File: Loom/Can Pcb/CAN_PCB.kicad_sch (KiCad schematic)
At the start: 28 parts, among them J1 Conn_01x02, J12 Conn_01x03, J15 Conn_01x03, J16 Conn_01x03, J2 Conn_01x05_Pin, J4 Conn_01x02, J5 Conn_01x03, U2 MCP2551-I-P, U4 TL780-05KCS, Y1 Crystal

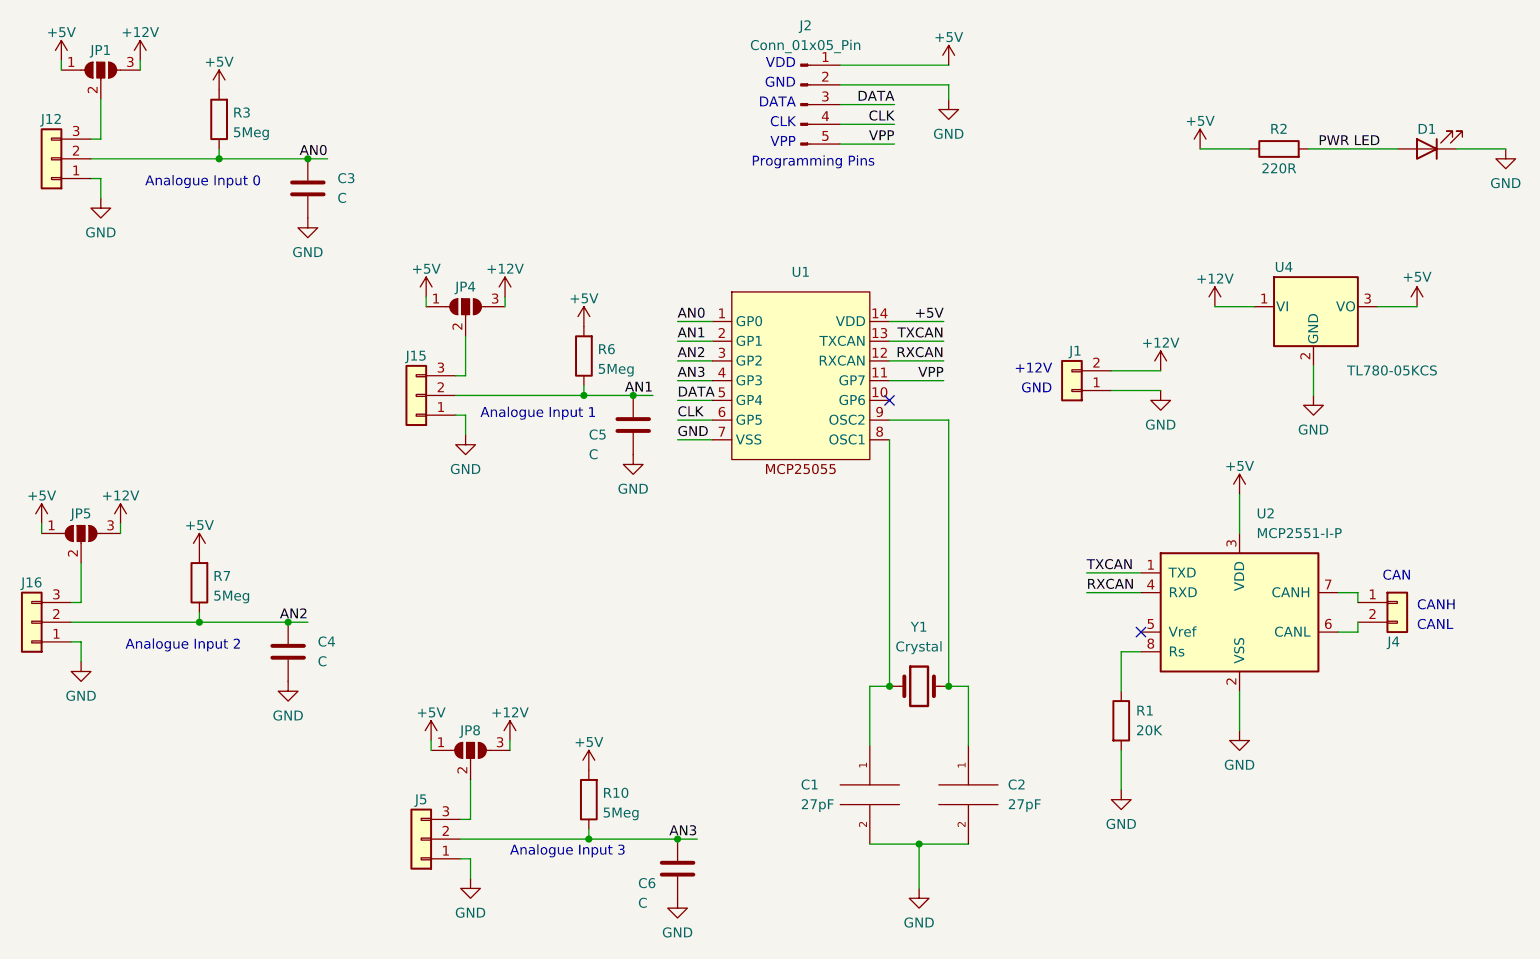
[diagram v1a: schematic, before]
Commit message: Revert "Merge branch 'CAN_PCB' of https://github.com/Full-Blue-Racing/FBR24-Electronics into CAN_PCB"
This reverts commit f7426b5fd5c3026a458d075125f69338a8895489, reversing
changes made to b85a40d8a8d15d08b24989522968470fc8db4cd4.
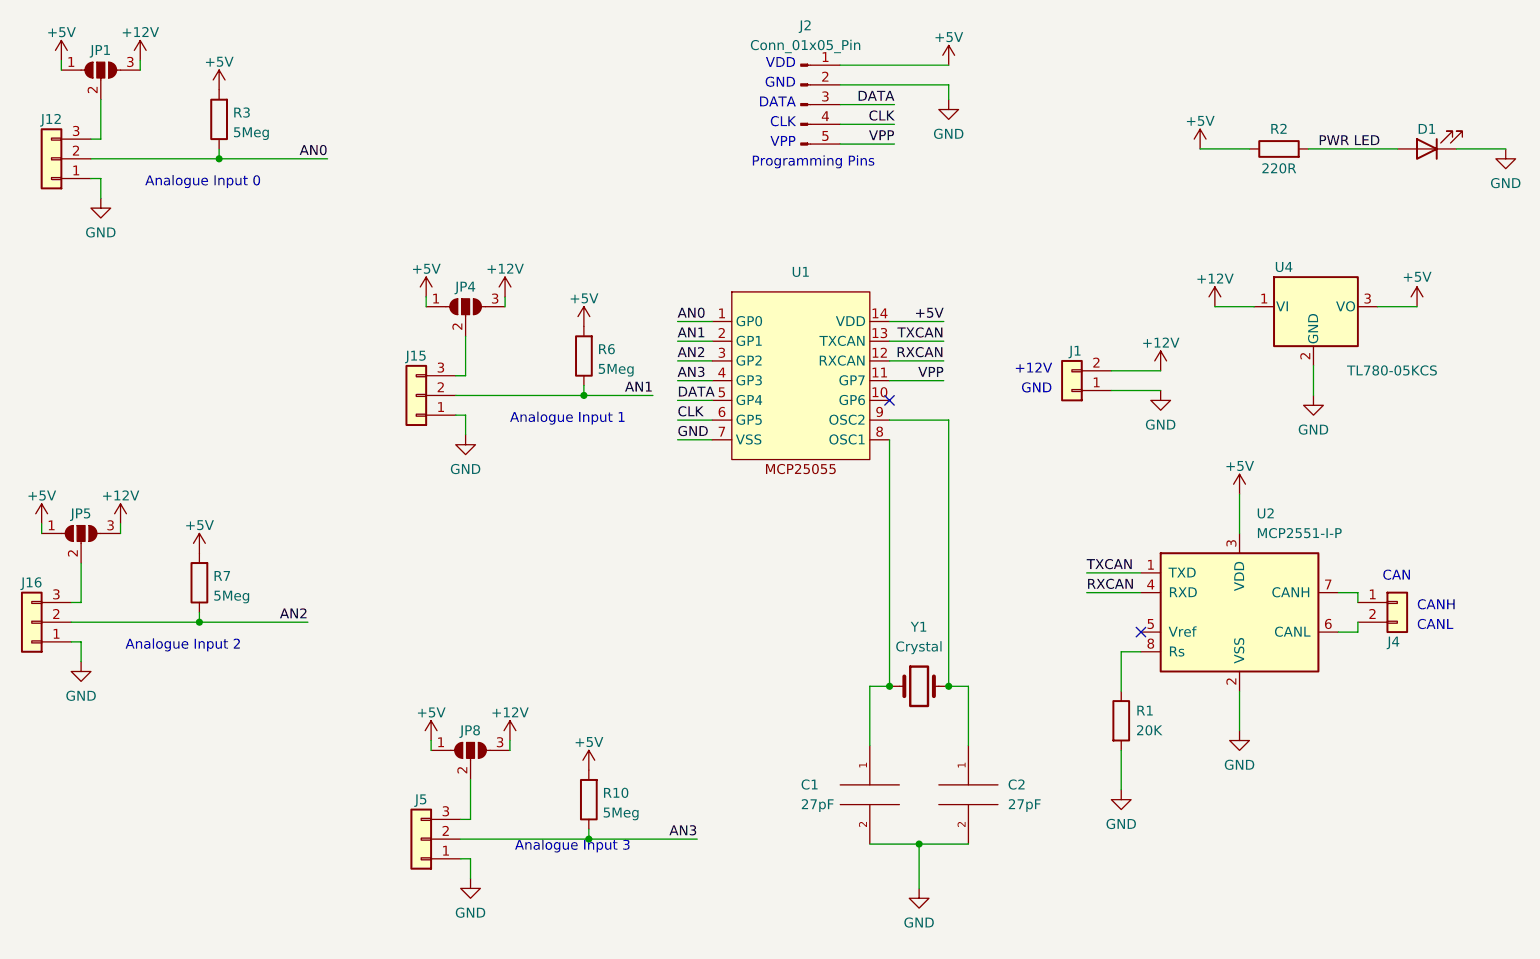
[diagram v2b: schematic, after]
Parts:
- removed C3, C4, C5, C6: C, Capacitor_THT:C_Disc_D4.7mm_W2.5mm_P5.00mm, symbol Device:C
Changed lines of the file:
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@@
     (title "Can Adapeter PCB")
   )
-  (junction (at 100.965 122.555) (diameter 0) (color 0 0 0 0)
-  )
   (junction (at 39.37 94.615) (diameter 0) (color 0 0 0 0)
   )
-  (junction (at 50.8 94.615) (diameter 0) (color 0 0 0 0)
-  )
   (junction (at 88.9 65.405) (diameter 0) (color 0 0 0 0)
   )
@@
   (junction (at 135.89 102.87) (diameter 0) (color 0 0 0 0)
   )
-  (junction (at 95.25 65.405) (diameter 0) (color 0 0 0 0)
-  )
   (junction (at 132.08 123.19) (diameter 0) (color 0 0 0 0)
-  )
-  (junction (at 53.34 34.925) (diameter 0) (color 0 0 0 0)
   )
   (junction (at 41.91 34.925) (diameter 0) (color 0 0 0 0)
@@
     (stroke (width 0) (type default))
   )
-  (wire (pts (xy 100.965 122.555) (xy 103.505 122.555))
-    (stroke (width 0) (type default))
-  )
   (wire (pts (xy 156.845 64.77) (xy 163.195 64.77))
     (stroke (width 0) (type default))
   )
-  (wire (pts (xy 95.25 65.405) (xy 97.79 65.405))
-    (stroke (width 0) (type default))
-  )
   (wire (pts (xy 100.965 68.58) (xy 105.41 68.58))
     (stroke (width 0) (type default))
@@
     (stroke (width 0) (type default))
   )
-  (wire (pts (xy 39.37 94.615) (xy 50.8 94.615))
+  (wire (pts (xy 39.37 94.615) (xy 53.34 94.615))
     (stroke (width 0) (type default))
   )
@@
     (stroke (width 0) (type default))
   )
-  (wire (pts (xy 88.9 65.405) (xy 95.25 65.405))
+  (wire (pts (xy 88.9 65.405) (xy 97.79 65.405))
     (stroke (width 0) (type default))
   )
@@
     (stroke (width 0) (type default))
   )
-  (wire (pts (xy 50.8 94.615) (xy 53.34 94.615))
-    (stroke (width 0) (type default))
-  )
   (wire (pts (xy 182.245 33.655) (xy 193.675 33.655))
     (stroke (width 0) (type default))
@@
     (stroke (width 0) (type default))
   )
-  (wire (pts (xy 53.34 34.925) (xy 55.88 34.925))
-    (stroke (width 0) (type default))
-  )
   (wire (pts (xy 121.92 30.48) (xy 128.905 30.48))
     (stroke (width 0) (type default))
@@
     (stroke (width 0) (type default))
   )
-  (wire (pts (xy 41.91 34.925) (xy 53.34 34.925))
-    (stroke (width 0) (type default))
-  )
-  (wire (pts (xy 89.535 122.555) (xy 100.965 122.555))
+  (wire (pts (xy 41.91 34.925) (xy 55.88 34.925))
+    (stroke (width 0) (type default))
+  )
+  (wire (pts (xy 89.535 122.555) (xy 103.505 122.555))
     (stroke (width 0) (type default))
   )
@@
     (effects (font (size 1.27 1.27)) (justify left bottom))
   )
-  (text "Analogue Input 3\n\n" (at 79.375 127 0)
+  (text "Analogue Input 3\n\n" (at 80.01 126.365 0)
     (effects (font (size 1.27 1.27)) (justify left bottom))
   )
@@
     (effects (font (size 1.27 1.27)) (justify right bottom))
   )
-  (text "Analogue Input 1\n" (at 75.565 68.58 0)
+  (text "Analogue Input 1\n" (at 79.375 69.215 0)
     (effects (font (size 1.27 1.27)) (justify left bottom))
   )
@@
     )
   )
-  (symbol (lib_id "Device:C") (at 95.25 69.215 0) (unit 1)
-    (in_bom yes) (on_board yes) (dnp no)
-    (property "Reference" "C5" (at 89.535 70.485 0)
-      (effects (font (size 1.27 1.27)) (justify left))
-    )
-    (property "Value" "C" (at 89.535 73.025 0)
-      (effects (font (size 1.27 1.27)) (justify left))
-    )
-    (property "Footprint" "Capacitor_THT:C_Disc_D4.7mm_W2.5mm_P5.00mm" (at 96.2152 73.025 0)
-      (effects (font (size 1.27 1.27)) hide)
-    )
-    (property "Datasheet" "~" (at 95.25 69.215 0)
-      (effects (font (size 1.27 1.27)) hide)
-    )
-    (pin "1")
-    (pin "2")
-    (instances
-      (project "CAN_PCB"
-        (path "/10118a9c-eb72-4c5f-b0c0-2b860c31ebad"
-          (reference "C5") (unit 1)
-        )
-      )
-    )
-  )
   (symbol (lib_id "power:+12V") (at 170.18 53.975 0) (unit 1)
     (in_bom yes) (on_board yes) (dnp no) (fields_autoplaced)
@@
     )
   )
-  (symbol (lib_id "power:GND") (at 53.34 42.545 0) (unit 1)
-    (in_bom yes) (on_board yes) (dnp no) (fields_autoplaced)
-    (property "Reference" "#PWR018" (at 53.34 48.895 0)
-      (effects (font (size 1.27 1.27)) hide)
-    )
-    (property "Value" "GND" (at 53.34 46.99 0)
-      (effects (font (size 1.27 1.27)))
-    )
-    (property "Footprint" "" (at 53.34 42.545 0)
-      (effects (font (size 1.27 1.27)) hide)
-    )
-    (property "Datasheet" "" (at 53.34 42.545 0)
-      (effects (font (size 1.27 1.27)) hide)
-    )
-    (pin "1")
-    (instances
-      (project "CAN_PCB"
-        (path "/10118a9c-eb72-4c5f-b0c0-2b860c31ebad"
-          (reference "#PWR018") (unit 1)
-        )
-      )
-    )
-  )
-  (symbol (lib_id "Device:C") (at 100.965 126.365 0) (unit 1)
-    (in_bom yes) (on_board yes) (dnp no)
-    (property "Reference" "C6" (at 95.885 128.27 0)
-      (effects (font (size 1.27 1.27)) (justify left))
-    )
-    (property "Value" "C" (at 95.885 130.81 0)
-      (effects (font (size 1.27 1.27)) (justify left))
-    )
-    (property "Footprint" "Capacitor_THT:C_Disc_D4.7mm_W2.5mm_P5.00mm" (at 101.9302 130.175 0)
-      (effects (font (size 1.27 1.27)) hide)
-    )
-    (property "Datasheet" "~" (at 100.965 126.365 0)
-      (effects (font (size 1.27 1.27)) hide)
-    )
-    (pin "1")
-    (pin "2")
-    (instances
-      (project "CAN_PCB"
-        (path "/10118a9c-eb72-4c5f-b0c0-2b860c31ebad"
-          (reference "C6") (unit 1)
-        )
-      )
-    )
-  )
   (symbol (lib_id "power:+12V") (at 31.75 22.225 0) (unit 1)
     (in_bom yes) (on_board yes) (dnp no) (fields_autoplaced)
@@
         (path "/10118a9c-eb72-4c5f-b0c0-2b860c31ebad"
           (reference "#PWR025") (unit 1)
-        )
-      )
-    )
-  )
-  (symbol (lib_id "power:GND") (at 50.8 102.235 0) (unit 1)
-    (in_bom yes) (on_board yes) (dnp no) (fields_autoplaced)
-    (property "Reference" "#PWR019" (at 50.8 108.585 0)
-      (effects (font (size 1.27 1.27)) hide)
-    )
-    (property "Value" "GND" (at 50.8 106.68 0)
-      (effects (font (size 1.27 1.27)))
-    )
-    (property "Footprint" "" (at 50.8 102.235 0)
-      (effects (font (size 1.27 1.27)) hide)
-    )
-    (property "Datasheet" "" (at 50.8 102.235 0)
-      (effects (font (size 1.27 1.27)) hide)
-    )
-    (pin "1")
-    (instances
-      (project "CAN_PCB"
-        (path "/10118a9c-eb72-4c5f-b0c0-2b860c31ebad"
-          (reference "#PWR019") (unit 1)
-        )
-      )
-    )
-  )
-  (symbol (lib_id "power:GND") (at 95.25 73.025 0) (unit 1)
-    (in_bom yes) (on_board yes) (dnp no) (fields_autoplaced)
-    (property "Reference" "#PWR017" (at 95.25 79.375 0)
-      (effects (font (size 1.27 1.27)) hide)
-    )
-    (property "Value" "GND" (at 95.25 77.47 0)
-      (effects (font (size 1.27 1.27)))
-    )
-    (property "Footprint" "" (at 95.25 73.025 0)
-      (effects (font (size 1.27 1.27)) hide)
-    )
-    (property "Datasheet" "" (at 95.25 73.025 0)
-      (effects (font (size 1.27 1.27)) hide)
-    )
-    (pin "1")
-    (instances
-      (project "CAN_PCB"
-        (path "/10118a9c-eb72-4c5f-b0c0-2b860c31ebad"
-          (reference "#PWR017") (unit 1)
-        )
-      )
-    )
-  )
-  (symbol (lib_id "power:GND") (at 100.965 130.175 0) (unit 1)
-    (in_bom yes) (on_board yes) (dnp no) (fields_autoplaced)
-    (property "Reference" "#PWR016" (at 100.965 136.525 0)
-      (effects (font (size 1.27 1.27)) hide)
-    )
-    (property "Value" "GND" (at 100.965 134.62 0)
-      (effects (font (size 1.27 1.27)))
-    )
-    (property "Footprint" "" (at 100.965 130.175 0)
-      (effects (font (size 1.27 1.27)) hide)
-    )
-    (property "Datasheet" "" (at 100.965 130.175 0)
-      (effects (font (size 1.27 1.27)) hide)
-    )
-    (pin "1")
-    (instances
-      (project "CAN_PCB"
-        (path "/10118a9c-eb72-4c5f-b0c0-2b860c31ebad"
-          (reference "#PWR016") (unit 1)
         )
       )
@@
         (path "/10118a9c-eb72-4c5f-b0c0-2b860c31ebad"
           (reference "#PWR041") (unit 1)
-        )
-      )
-    )
-  )
-  (symbol (lib_id "Device:C") (at 53.34 38.735 0) (unit 1)
-    (in_bom yes) (on_board yes) (dnp no) (fields_autoplaced)
-    (property "Reference" "C3" (at 57.15 37.465 0)
-      (effects (font (size 1.27 1.27)) (justify left))
-    )
-    (property "Value" "C" (at 57.15 40.005 0)
-      (effects (font (size 1.27 1.27)) (justify left))
-    )
-    (property "Footprint" "Capacitor_THT:C_Disc_D4.7mm_W2.5mm_P5.00mm" (at 54.3052 42.545 0)
-      (effects (font (size 1.27 1.27)) hide)
-    )
-    (property "Datasheet" "~" (at 53.34 38.735 0)
-      (effects (font (size 1.27 1.27)) hide)
-    )
-    (pin "1")
-    (pin "2")
-    (instances
-      (project "CAN_PCB"
-        (path "/10118a9c-eb72-4c5f-b0c0-2b860c31ebad"
-          (reference "C3") (unit 1)
         )
       )
@@
         )
       )
-    )
-  )
-  (symbol (lib_id "Device:C") (at 50.8 98.425 0) (unit 1)
-    (in_bom yes) (on_board yes) (dnp no) (fields_autoplaced)
-    (property "Reference" "C4" (at 54.61 97.155 0)
-      (effects (font (size 1.27 1.27)) (justify left))
-    )
-    (property "Value" "C" (at 54.61 99.695 0)
-      (effects (font (size 1.27 1.27)) (justify left))
-    )
-    (property "Footprint" "Capacitor_THT:C_Disc_D4.7mm_W2.5mm_P5.00mm" (at 51.7652 102.235 0)
-      (effects (font (size 1.27 1.27)) hide)
-    )
-    (property "Datasheet" "~" (at 50.8 98.425 0)
-      (effects (font (size 1.27 1.27)) hide)
-    )
-    (pin "1")
-    (pin "2")
-    (instances
-      (project "CAN_PCB"
-        (path "/10118a9c-eb72-4c5f-b0c0-2b860c31ebad"
-          (reference "C4") (unit 1)
-        )
-      )
